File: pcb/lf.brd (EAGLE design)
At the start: 160 x 27.6 mm, 49 parts, among them IC1 TB6612FNG, U1 STM32F103RBT6, X1 FH12-14S-0.5SH

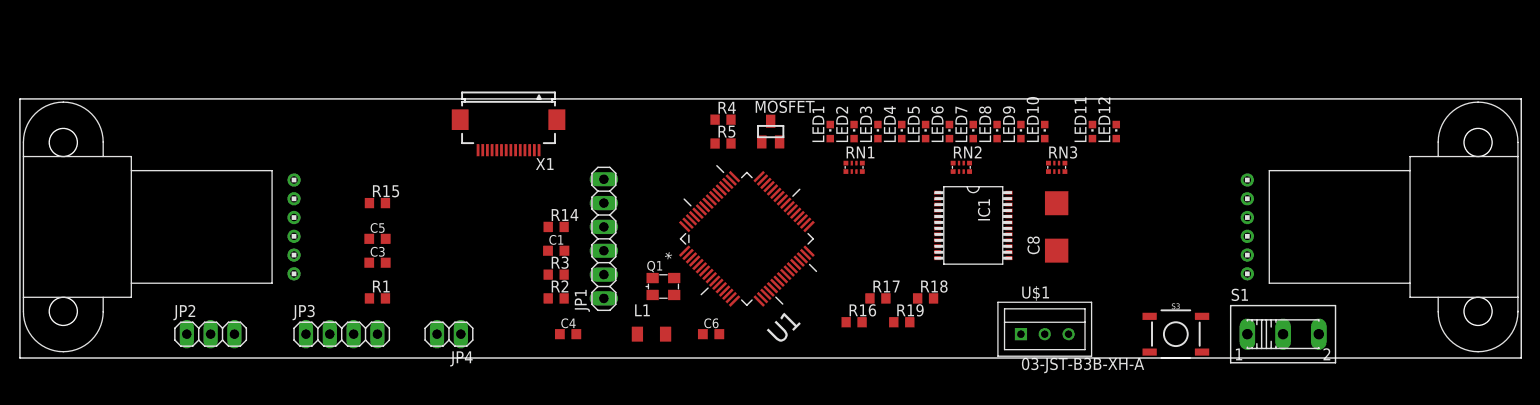
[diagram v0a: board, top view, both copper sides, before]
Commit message: o już niewiele
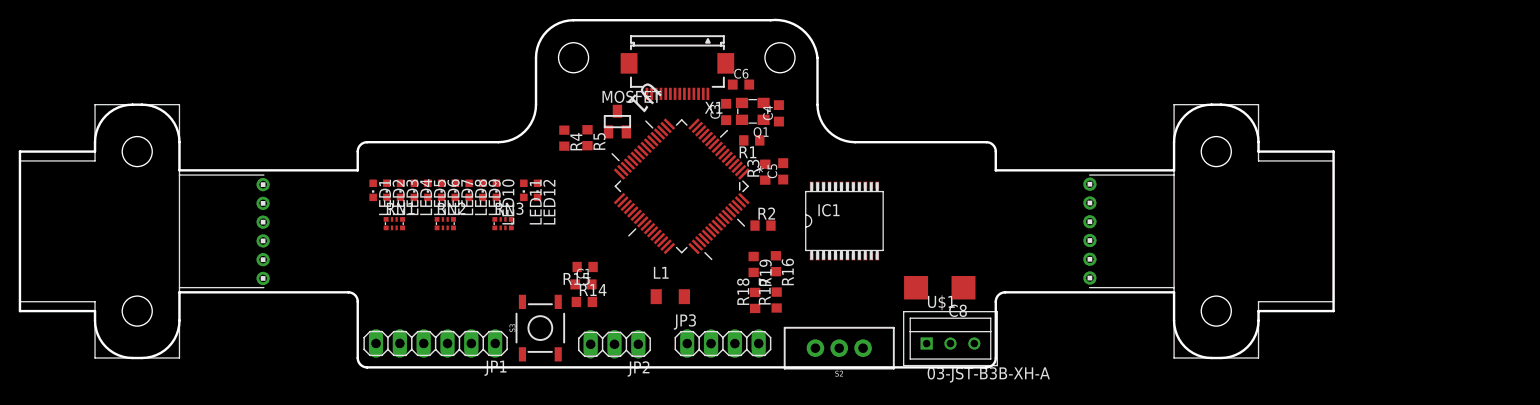
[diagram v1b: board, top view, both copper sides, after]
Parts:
- removed JP4: (no value), pinhead:1X02
- removed S1: (no value), switch:255SB
- removed U$2, U$3: (no value), PololuMG_v2:HP_NM
- added S2: (no value), SparkFun-Switches:SWITCH_SPDT_PTH_11.6X4.0MM
- moved S3 67.7 mm to (55.5, 3.19), turned to 90 degrees
- moved LED12 62.0 mm to (55.2, 17.9), turned to 180 degrees
- moved LED11 60.9 mm to (53.7, 17.9), turned to 180 degrees
- moved RN3 59.3 mm to (51.5, 14.3)
- moved LED10 58.8 mm to (50.8, 17.9), turned to 180 degrees
- moved LED9 57.7 mm to (49.3, 17.9), turned to 180 degrees
- moved LED8 56.6 mm to (47.9, 17.9), turned to 180 degrees
- moved LED7 55.6 mm to (46.4, 17.9), turned to 180 degrees
- moved RN2 55.3 mm to (45.3, 14.3)
- moved LED6 54.5 mm to (44.9, 17.9), turned to 180 degrees
- moved LED5 53.4 mm to (43.5, 17.9), turned to 180 degrees
- moved LED4 52.3 mm to (42.0, 17.9), turned to 180 degrees
- moved LED3 51.3 mm to (40.6, 17.9), turned to 180 degrees
- moved LED2 50.2 mm to (39.1, 17.9), turned to 180 degrees
- moved RN1 49.4 mm to (39.9, 14.3)
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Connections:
- removed net N$13: R18.1, U$1.P$1
- net GND: no longer JP4.2
- net N$12: now also R18.1, S2.3, U$1.P$1; no longer JP4.1, S1.3
- net VMOT: now also S2.2; no longer S1.2
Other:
- board size 160 x 27.6 mm -> 140 x 37 mm
